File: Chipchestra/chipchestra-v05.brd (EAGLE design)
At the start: 40.9 x 59.7 mm, 14 parts

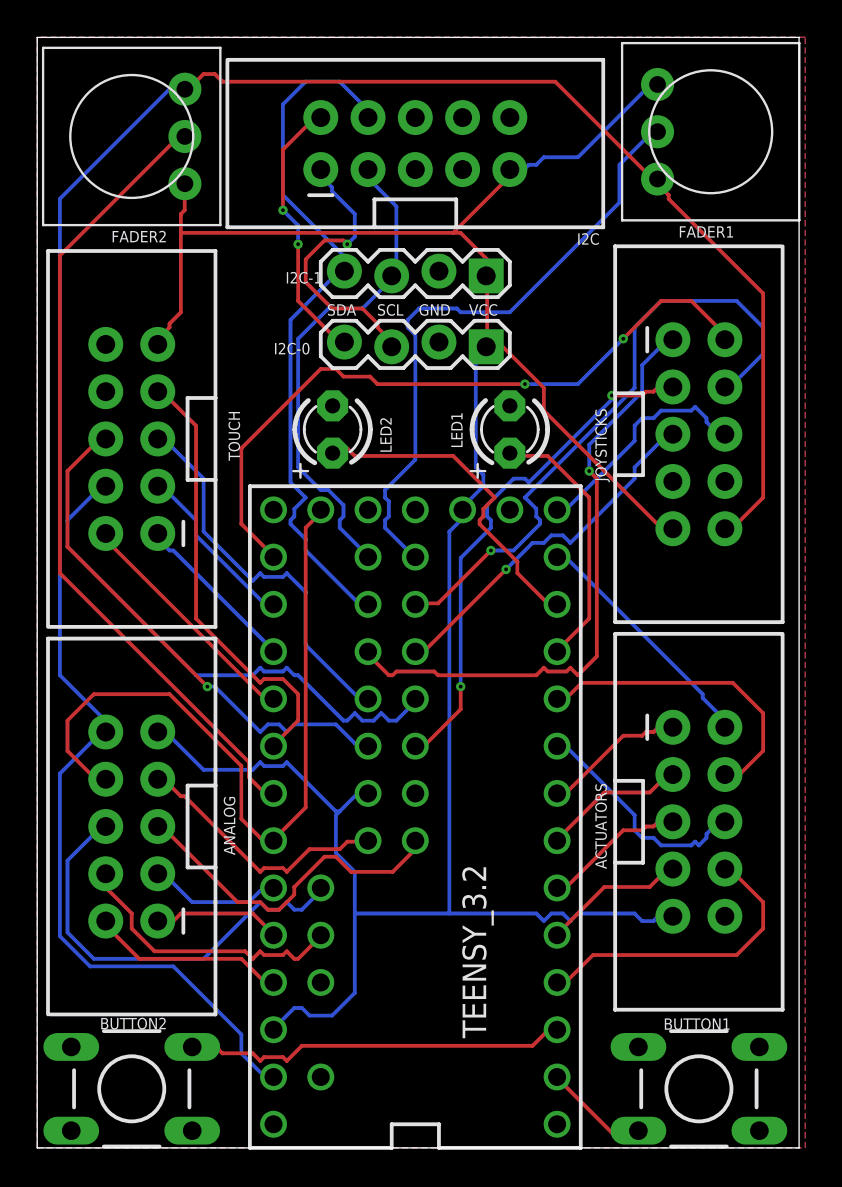
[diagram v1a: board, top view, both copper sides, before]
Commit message: many changes to chipchestra
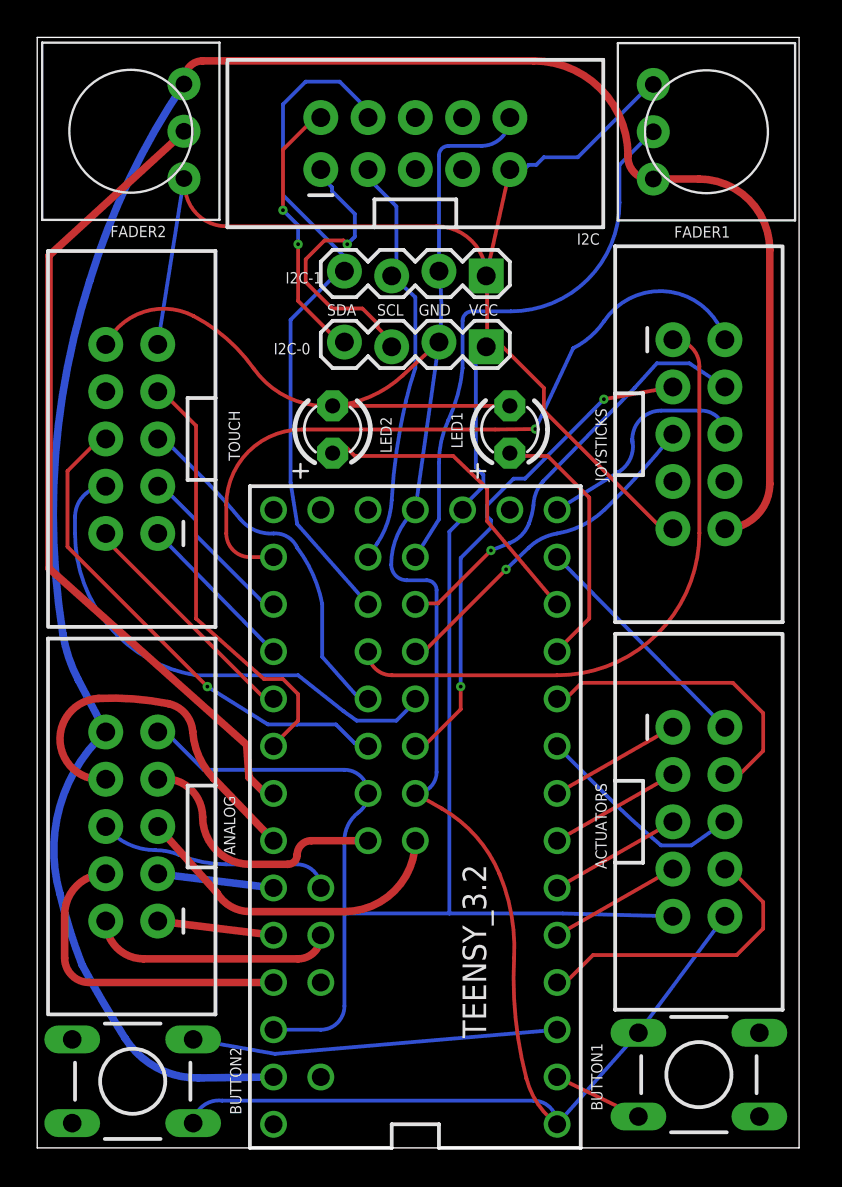
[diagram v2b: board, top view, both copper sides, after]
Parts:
- moved BUTTON1 0.76 mm to (35.6, 3.94)
- moved BUTTON2 0.41 mm to (5.13, 3.58)
- moved FADER2 0.28 mm to (5.03, 54.6)
- moved FADER1 0.23 mm to (36.0, 54.6)
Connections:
- new net DAC: TEENSY_3.2.RESET/DAC
- new net N$1: TEENSY_3.2.13
- net ANALOG2: now also TEENSY_3.2.A10; no longer TEENSY_3.2.23/A9
- net ANALOG4: now also TEENSY_3.2.23/A9; no longer TEENSY_3.2.A10
- net ANALOG8: no longer TEENSY_3.2.RESET/DAC
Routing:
- net GND: track 0.00 -> 126.9 mm
- net ANALOG8: track 39.8 -> 17.5 mm
- net JOYH2: track 34.2 -> 23.1 mm
- net ANALOG6: track 23.2 -> 12.4 mm
- net FADER1: track 33.6 -> 29.3 mm
- net I2C_SCL1: track 26.7 -> 22.5 mm
- net ANALOG2: track 10.6 -> 13.0 mm
- net TOUCH4: track 28.6 -> 26.4 mm
- net ANALOG4: track 15.4 -> 17.2 mm
- net TOUCH5: track 21.0 -> 19.4 mm
- net AGND: track 116.5 -> 115.0 mm
- net FADER2: track 43.3 -> 44.6 mm
- net I2C_SDA1: track 38.4 -> 37.3 mm
- net BUTTON2: track 20.9 -> 19.7 mm
- net ANALOG5: track 18.4 -> 17.3 mm
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- removed copper zone on layer 1, net GND
- removed copper zone on layer 16, net GND
